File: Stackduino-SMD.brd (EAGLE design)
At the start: 62.5 x 68 mm, 65 parts

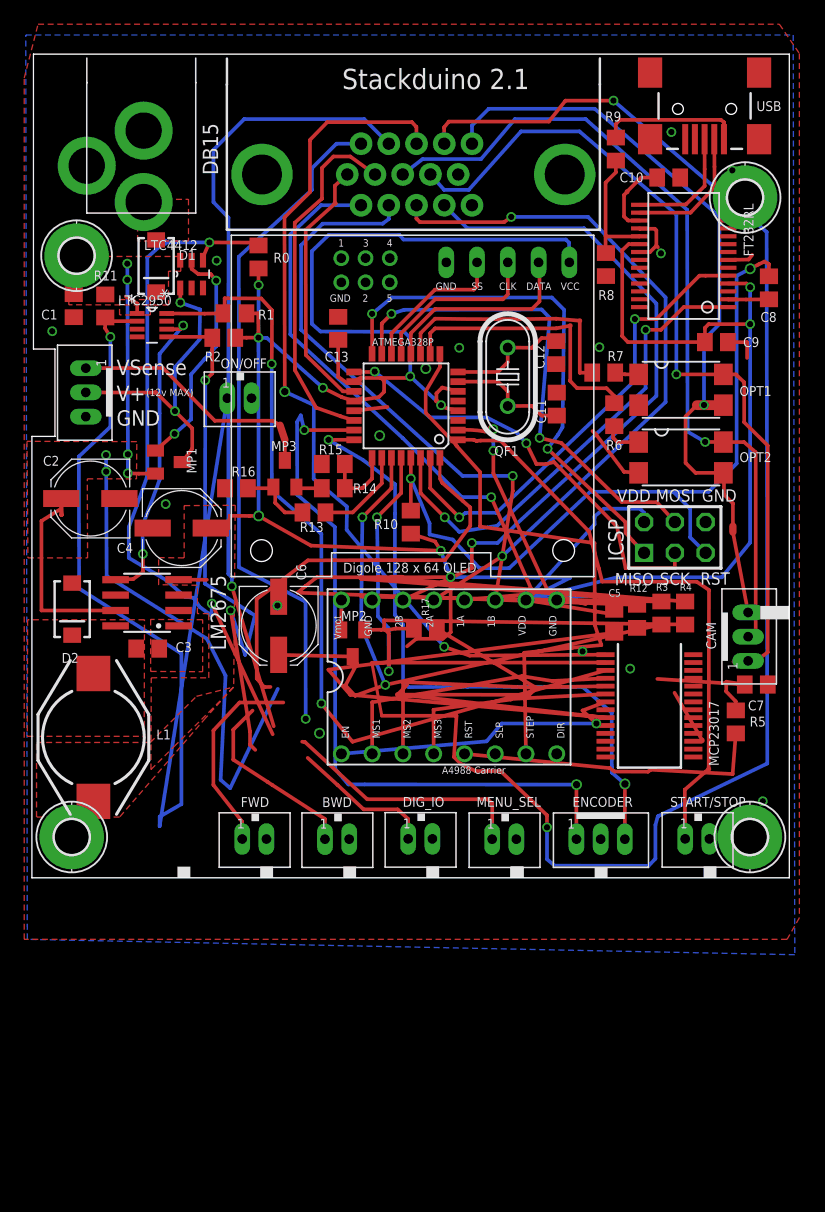
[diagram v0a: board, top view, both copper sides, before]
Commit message: latest progress on brd v2.1
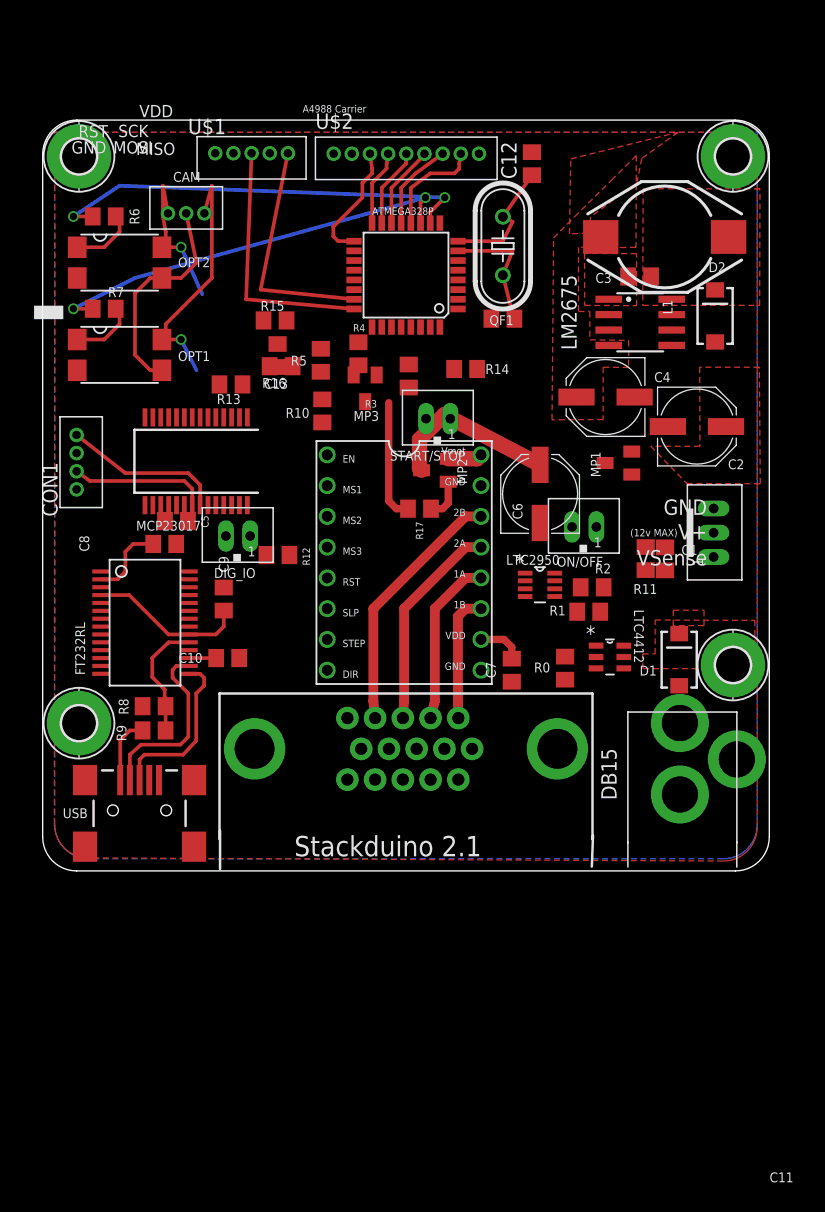
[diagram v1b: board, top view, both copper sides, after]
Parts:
- removed BWD, FWD, MENU_SEL: JST-PH_2-PIN_HEADER, SRG:JST_B2B-PH_HEADER
- removed ENCODER: JST-PH_3-PIN_HEADER, SRG:JST_B3B-PH_HEADER
- removed ICSP: AVR-ISP-6, avr-5:AVR-ISP-6
- added CON1: B4B-ZR, jst-connectors:B4B-ZR
- added U$1: B5B-ZR, jst-connectors:B5B-ZR
- CAM: value JST-PH_3-PIN_HEADER -> B3B-ZR; device SRG:JST_B3B-PH_HEADER -> jst-connectors:B3B-ZR
- U$2: value OLED Display -> B9B-ZR; device Stackduino:DIGOLE_OLED -> jst-connectors:B9B-ZR
- moved H2 78.9 mm to (3.00, 71.0), turned to 180 degrees
- moved H1 78.4 mm to (57.0, 71.0), turned to 180 degrees
- moved 12VDC 76.0 mm to (52.7, 14.9), turned to 180 degrees
- moved USB 74.4 mm to (8.00, 17.0), turned to 90 degrees
- moved H4 70.1 mm to (3.00, 24.2), turned to 180 degrees
- moved H3 63.9 mm to (57.0, 29.0), turned to 180 degrees
- moved L1 62.7 mm to (51.4, 64.3), turned to 180 degrees
- moved R9 61.3 mm to (9.20, 23.6), turned to 0 degrees
- moved D2 58.3 mm to (55.5, 57.8), turned to 90 degrees
- moved CAM 58.0 mm to (11.8, 66.3), turned to 180 degrees
- moved DB15 57.6 mm to (30.0, 17.0), turned to 180 degrees
- moved C8 54.2 mm to (10.1, 39.0), turned to 180 degrees
- moved D1 54.1 mm to (52.6, 29.4), turned to 90 degrees
- moved C10 53.9 mm to (15.3, 29.6)
- moved FT232RL 53.8 mm to (8.45, 32.5), turned to 270 degrees
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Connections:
- removed net N$11: ATMEGA328P.29, C8.1, ICSP.5, R10.1
- new net +5V: U$2.9
- new net RESET: ATMEGA328P.29, C8.1, R10.1, U$2.8
- net BWD: now also CON1.1; no longer BWD.P1
- net CAM_GND: now also CAM.2; no longer CAM.P3
- net ENCSWITCH: now also U$1.5; no longer MENU_SEL.P1
- net ENC_A: now also U$1.1; no longer ENCODER.P1
- net ENC_B: now also U$1.3; no longer ENCODER.P3
- net FWD: now also CON1.3; no longer FWD.P1
- net GND: now also CON1.2, CON1.4, U$1.2, U$1.4, U$2.1; no longer BWD.P2, ENCODER.P2, FWD.P2, ICSP.6, MENU_SEL.P2, U$2.GND@1, U$2.GND@2
- net MISO: now also U$2.6; no longer ICSP.1
- net MOSI: now also U$2.5; no longer ICSP.4
- net N$22: now also U$2.4; no longer U$2.SS
- net N$23: now also U$2.2; no longer U$2.DATA
- net N$24: now also U$2.3; no longer U$2.CLK
- net OPT1: now also CAM.3; no longer CAM.P2
- net OPT2: now also CAM.1; no longer CAM.P1
- net OUT1A: now also A4988_CARRIER.1B; no longer A4988_CARRIER.1A
- net OUT1B: now also A4988_CARRIER.1A; no longer A4988_CARRIER.1B
- net SCK: now also U$2.7; no longer ICSP.3
- net VCC: no longer ICSP.2, U$2.VCC
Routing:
- net VCC: track 457.0 -> 26.8 mm, vias 10 -> 0
- net DIG2: track 146.4 -> 0.00 mm, vias 2 -> 0
- net PBUTTON: track 87.4 -> 0.00 mm, vias 1 -> 0
- net DIG1: track 72.9 -> 0.00 mm, vias 2 -> 0
- net V+: track 86.9 -> 14.4 mm, vias 6 -> 0
- net KILL: track 70.4 -> 0.00 mm, vias 2 -> 0
- net LIM2: track 65.1 -> 0.00 mm, vias 1 -> 0
- net N$11: track 64.8 -> 0.00 mm, vias 2 -> 0
- net STAT: track 57.8 -> 0.00 mm, vias 2 -> 0
- net LIM1: track 56.4 -> 0.00 mm, vias 1 -> 0
- net OPT1: track 68.5 -> 13.8 mm
- net OPT2: track 72.0 -> 21.1 mm
- net N$19: track 49.4 -> 0.00 mm, vias 2 -> 0
- net STEP: track 49.1 -> 0.00 mm
- net CAM_GND: track 67.0 -> 18.1 mm, vias 1 -> 0
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- removed copper zone on layer 1, net VIN
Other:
- board size 62.5 x 68 mm -> 60 x 62 mm
